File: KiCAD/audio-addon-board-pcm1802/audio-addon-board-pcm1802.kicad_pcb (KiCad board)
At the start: 2 copper layers, 85 x 30.5 mm, 68 parts, among them J1 RCA, J2 CONN_HOST_1, J3 RCA, J4 RCA, J5 RCA, SW1 SW_DIP_x04, U1 PCM1802DBR, U2 LTC1682IS8-5, U3 SN74LVC1G125DBV

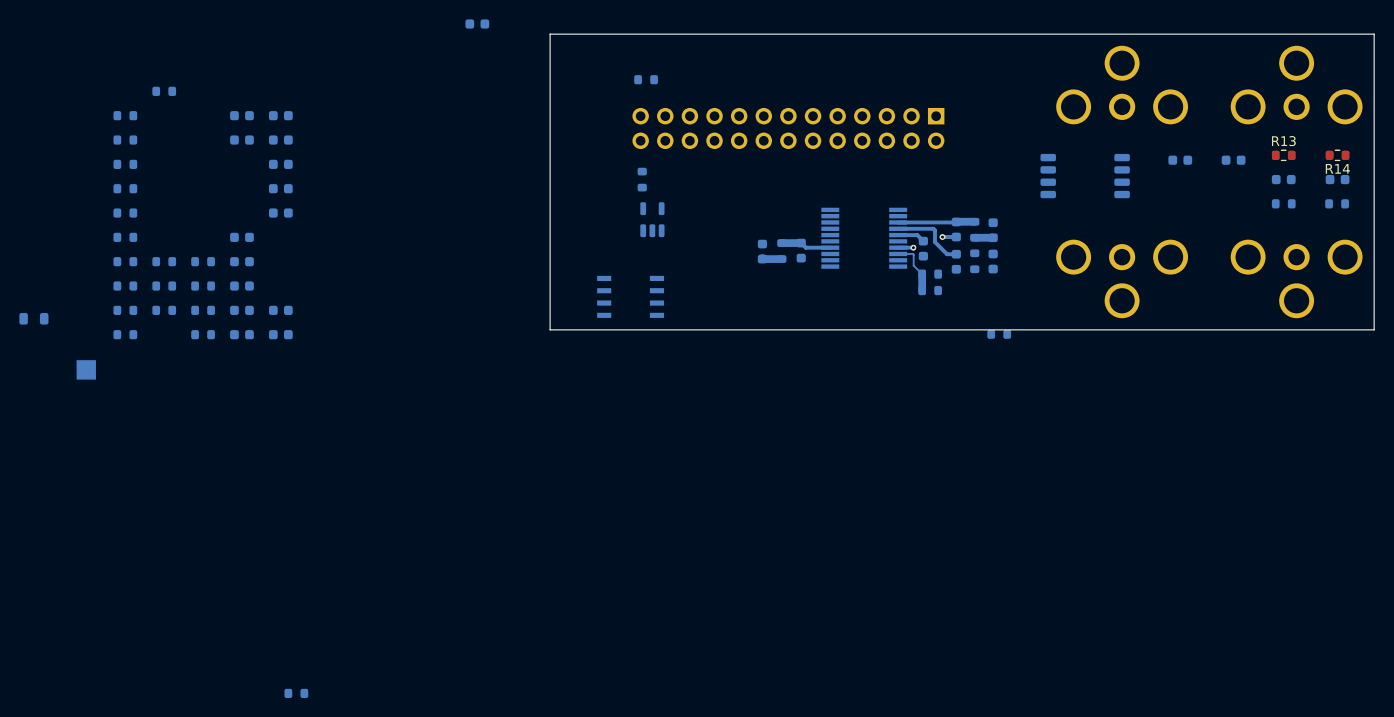
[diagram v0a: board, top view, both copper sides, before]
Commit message: working on layout
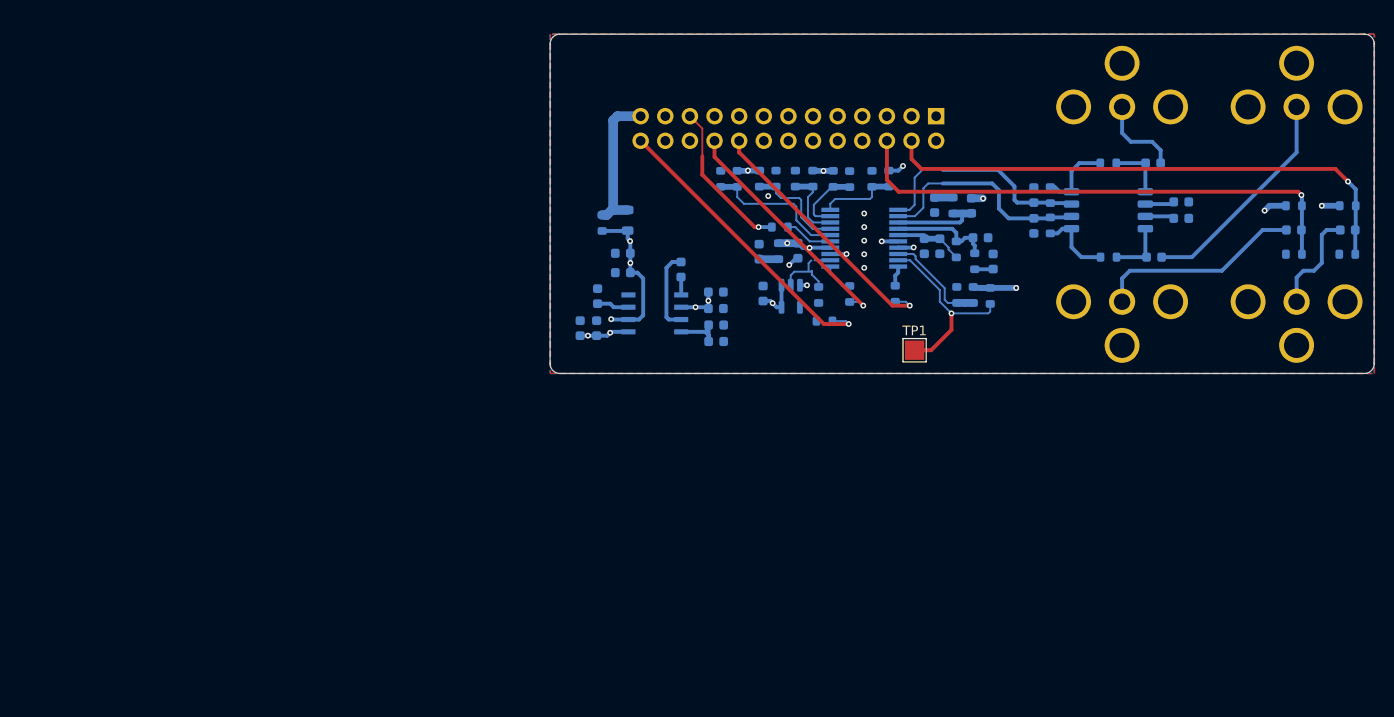
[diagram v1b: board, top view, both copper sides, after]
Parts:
- added C25: 1uF, Capacitor_SMD:C_0603_1608Metric, B.Cu at (122.0, 76.8)
- R13, R14: moved to B.Cu
- TP1: moved to F.Cu
- moved RA3 98.2 mm to (157.6, 63.3)
- moved RA4 97.6 mm to (157.6, 73.0)
- moved C21 97.3 mm to (165.1, 69.0), turned to 0 degrees
- moved C20 97.3 mm to (165.1, 67.3), turned to 0 degrees
- moved RA2 91.5 mm to (151.6, 69.7), turned to 90 degrees
- moved R8 87.8 mm to (145.4, 77.0), turned to -90 degrees
- moved TP1 85.5 mm to (137.6, 82.6), turned to 0 degrees
- moved C18 81.8 mm to (149.9, 66.6), turned to -90 degrees
- moved C19 81.8 mm to (149.9, 69.8), turned to -90 degrees
- moved RMODE1 79.0 mm to (134.9, 64.9), turned to 90 degrees
- moved RMODE4 77.8 mm to (133.2, 64.9), turned to -90 degrees
- moved R4 77.7 mm to (141.9, 72.2), turned to 90 degrees
- moved RMODE2 75.2 mm to (130.9, 65.0), turned to -90 degrees
- moved RMODE0 73.1 mm to (129.2, 64.9), turned to -90 degrees
- moved R7 71.5 mm to (135.6, 76.8), turned to 90 degrees
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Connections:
- J1 pad 2: unconnected-(J1-Ext-Pad2) -> GND
- J4 pad 2: unconnected-(J4-Ext-Pad2) -> GND
- SW1 pad 1: Net-(C20-Pad1) -> Net-(C12-Pad2)
- SW1 pad 2: Net-(C12-Pad2) -> Net-(C20-Pad1)
- SW1 pad 3: Net-(C17-Pad2) -> Net-(C21-Pad1)
- SW1 pad 4: Net-(C21-Pad1) -> Net-(C17-Pad2)
- SW1 pad 5: VINR -> Net-(RA2-Pad1)
- SW1 pad 6: Net-(RA2-Pad1) -> VINR
- SW1 pad 7: Net-(RA1-Pad1) -> VINL
- SW1 pad 8: VINL -> Net-(RA1-Pad1)
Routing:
- net +3.3V: track 6.77 -> 83.1 mm, vias 1 -> 15
- net /+5V, Analog: track 2.86 -> 70.4 mm, vias 0 -> 2
- net Net-(J2-Pin_4): track 0.00 -> 55.7 mm, vias 0 -> 1
- net Net-(J2-Pin_6): track 0.00 -> 53.6 mm, vias 0 -> 1
- net DOUT: track 0.00 -> 31.1 mm, vias 0 -> 1
- net LRCK: track 0.00 -> 27.0 mm, vias 0 -> 1
- net BCK: track 0.00 -> 24.9 mm, vias 0 -> 1
- net VINL: track 0.00 -> 23.5 mm
- net VINR: track 0.00 -> 23.1 mm
- net Net-(J5-In): track 0.00 -> 23.1 mm
- net Net-(J1-In): track 0.00 -> 21.4 mm
- net Net-(U1-FSYNC): track 0.00 -> 19.7 mm, vias 0 -> 1
- net SCKI: track 0.00 -> 16.0 mm, vias 0 -> 1
- net /+3v3 from host: track 0.00 -> 15.1 mm
- net Net-(U1-OSR): track 0.00 -> 14.8 mm
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- added copper zone on In1.Cu, net +3.3V
- added copper zone on B.Cu, net GND
- added copper zone on F.Cu, net GND
- added copper zone on In2.Cu, net GND
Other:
- board size 85 x 30.5 mm -> 85 x 35 mm
- copper layers 2 -> 4
